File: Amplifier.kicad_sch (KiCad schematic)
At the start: 22 parts, among them Q1 BC547, Q2 2N3904

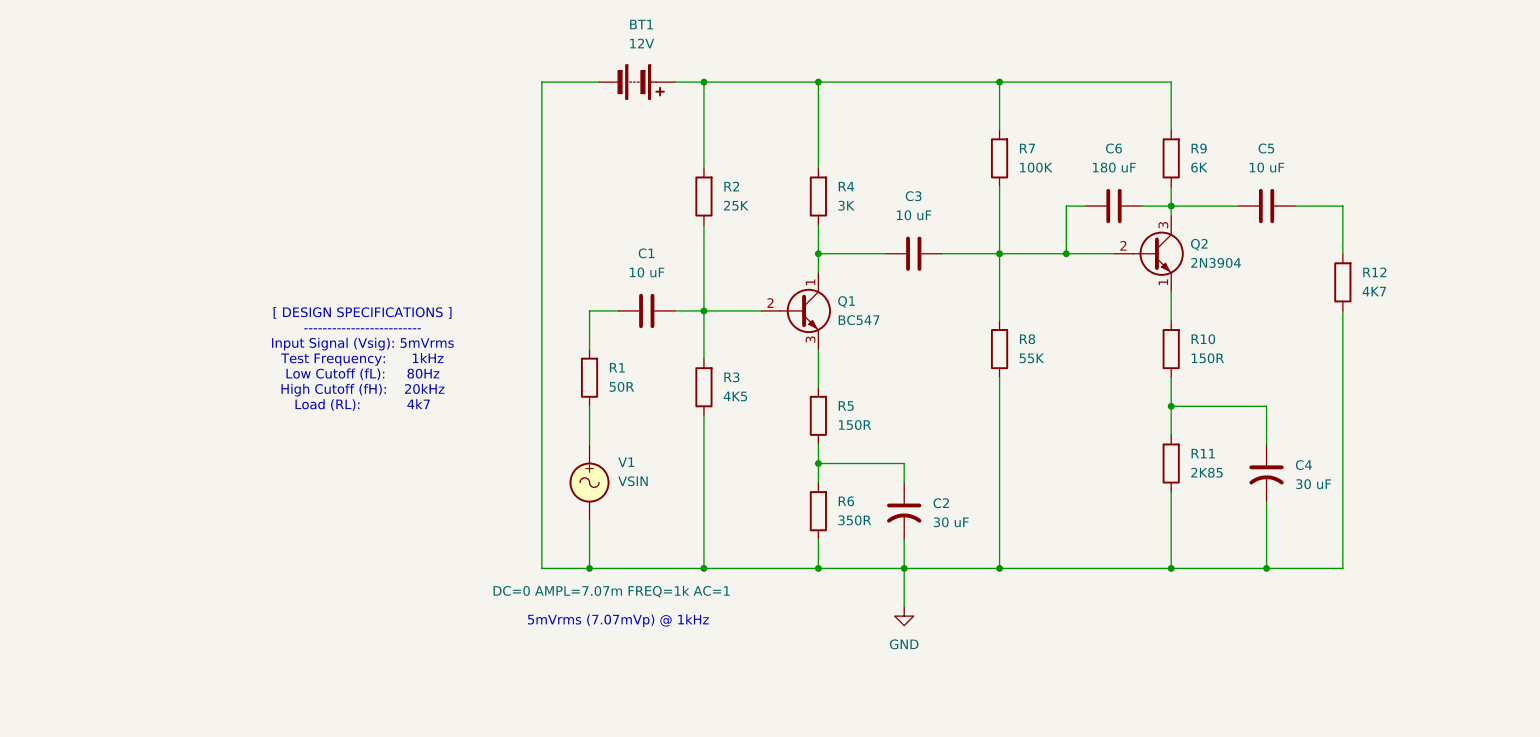
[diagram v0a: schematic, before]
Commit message: v2.0 3.24.2026
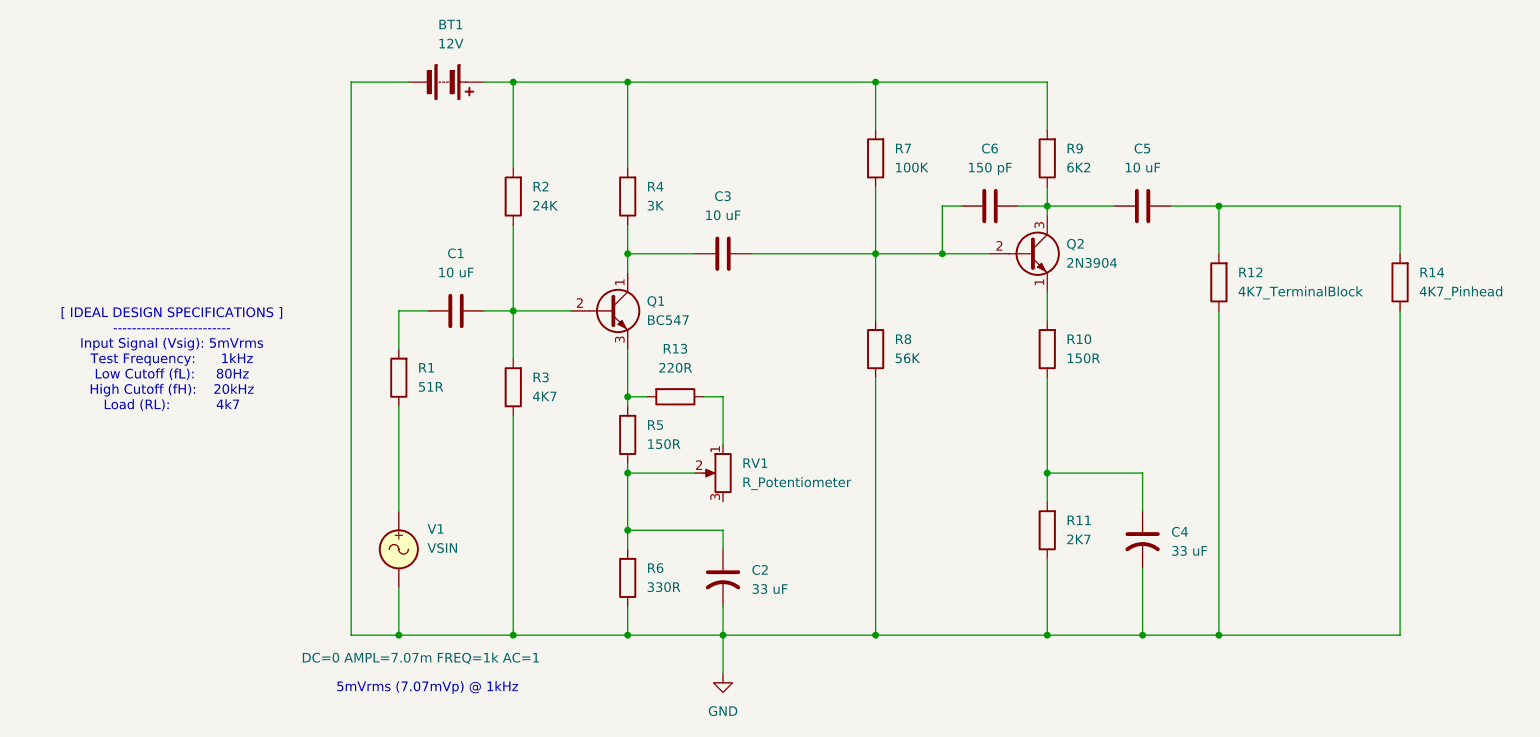
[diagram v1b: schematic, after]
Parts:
- added R13: 220R, Resistor_THT:R_Axial_DIN0207_L6.3mm_D2.5mm_P10.16mm_Horizontal, symbol Device:R
- added R14: 4K7_Pinhead, Connector_PinHeader_2.54mm:PinHeader_1x02_P2.54mm_Vertical, symbol Device:R
- added RV1: R_Potentiometer, TerminalBlock_Phoenix:TerminalBlock_Phoenix_MKDS-1,5-2_1x02_P5.00mm_Horizontal, symbol Device:R_Potentiometer
- C1, C3, C5: footprint Capacitor_THT:C_Disc_D5.1mm_W3.2mm_P5.00mm -> Capacitor_THT:C_Disc_D4.3mm_W1.9mm_P5.00mm
- C2, C4: value 30 uF -> 33 uF
- C6: value 180 uF -> 150 pF
- R1: value 50R -> 51R
- R11: value 2K85 -> 2K7
- R12: value 4K7 -> 4K7_TerminalBlock
- R2: value 25K -> 24K
- R3: value 4K5 -> 4K7
- R6: value 350R -> 330R
- R8: value 55K -> 56K
- R9: value 6K -> 6K2
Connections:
- net GND: now also R14.1
- net at Q1.3 (E), R5.2: now also R13.2
- net at C2.1, R5.1, R6.2: now also RV1.2
- net at C5.1, R12.2: now also R14.2
- new net: R13.1, RV1.1
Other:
- note added: "[ IDEAL DESIGN SPECIFICATIONS ] ------------------------- Input Signal (Vsig): 5mVrms Test Frequency: 1kHz Low Cutoff (fL): 80Hz High Cutoff (fH): 20kHz Load (RL): 4k7"
- note removed: "[ DESIGN SPECIFICATIONS ] ------------------------- Input Signal (Vsig): 5mVrms Test Frequency: 1kHz Low Cutoff (fL): 80Hz High Cutoff (fH): 20kHz Load (RL): 4k7"
- moved on the sheet: BT1, C1, C2, C3, C4, C5, C6, Q1, Q2, R1, R10, R11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
